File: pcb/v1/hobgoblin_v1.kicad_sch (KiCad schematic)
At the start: 45 parts, among them J1 5V, J2 RC2014EXT1, J3 RC2014EXT2, SW1 RESET, SW2 ROMBNK, U1 74LS32, U2 Z80CPU, U3 74LS14, U4 74LS138, U5 628128, U6 74LS32, U7 74HCT00, U8 SST39SF010, U9 MC68B50, X1 10MHz, X2 7.3728MHz

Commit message: Rename CF Card connector footprint to match the actual part
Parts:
- CF1: footprint hobgoblin:CF-Card_3M_N7E50-7516PK-20-WF -> hobgoblin:CF-Card_3M_N7E507516PK20
- U1: footprint (none) -> Package_DIP:DIP-14_W7.62mm_LongPads
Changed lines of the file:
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@@
     (property "Reference" "CF1" (id 0) (at 222.25 18.669 0))
     (property "Value" "CF_Socket" (id 1) (at 222.25 20.9804 0))
-    (property "Footprint" "hobgoblin:CF-Card_3M_N7E50-7516PK-20-WF" (id 2) (at 222.25 57.15 0)
+    (property "Footprint" "hobgoblin:CF-Card_3M_N7E507516PK20" (id 2) (at 222.25 57.15 0)
       (effects (font (size 1.27 1.27)) hide)
     )
@@
     (property "Reference" "U1" (id 0) (at 27.94 125.73 0))
     (property "Value" "74LS32" (id 1) (at 33.02 121.92 0))
-    (property "Footprint" "" (id 2) (at 27.94 125.73 0)
+    (property "Footprint" "Package_DIP:DIP-14_W7.62mm_LongPads" (id 2) (at 27.94 125.73 0)
       (effects (font (size 1.27 1.27)) hide)
     )
@@
     )
     (path "/00000000-0000-0000-0000-00005fec22e8"
-      (reference "CF1") (unit 1) (value "CF_Socket") (footprint "hobgoblin:CF-Card_3M_N7E50-7516PK-20-WF")
+      (reference "CF1") (unit 1) (value "CF_Socket") (footprint "hobgoblin:CF-Card_3M_N7E507516PK20")
     )
     (path "/00000000-0000-0000-0000-00005f8c4542"
@@
     )
     (path "/00000000-0000-0000-0000-0000600d80cc"
-      (reference "U1") (unit 2) (value "74LS32") (footprint "")
+      (reference "U1") (unit 2) (value "74LS32") (footprint "Package_DIP:DIP-14_W7.62mm_LongPads")
     )
     (path "/00000000-0000-0000-0000-00005fb5d442"

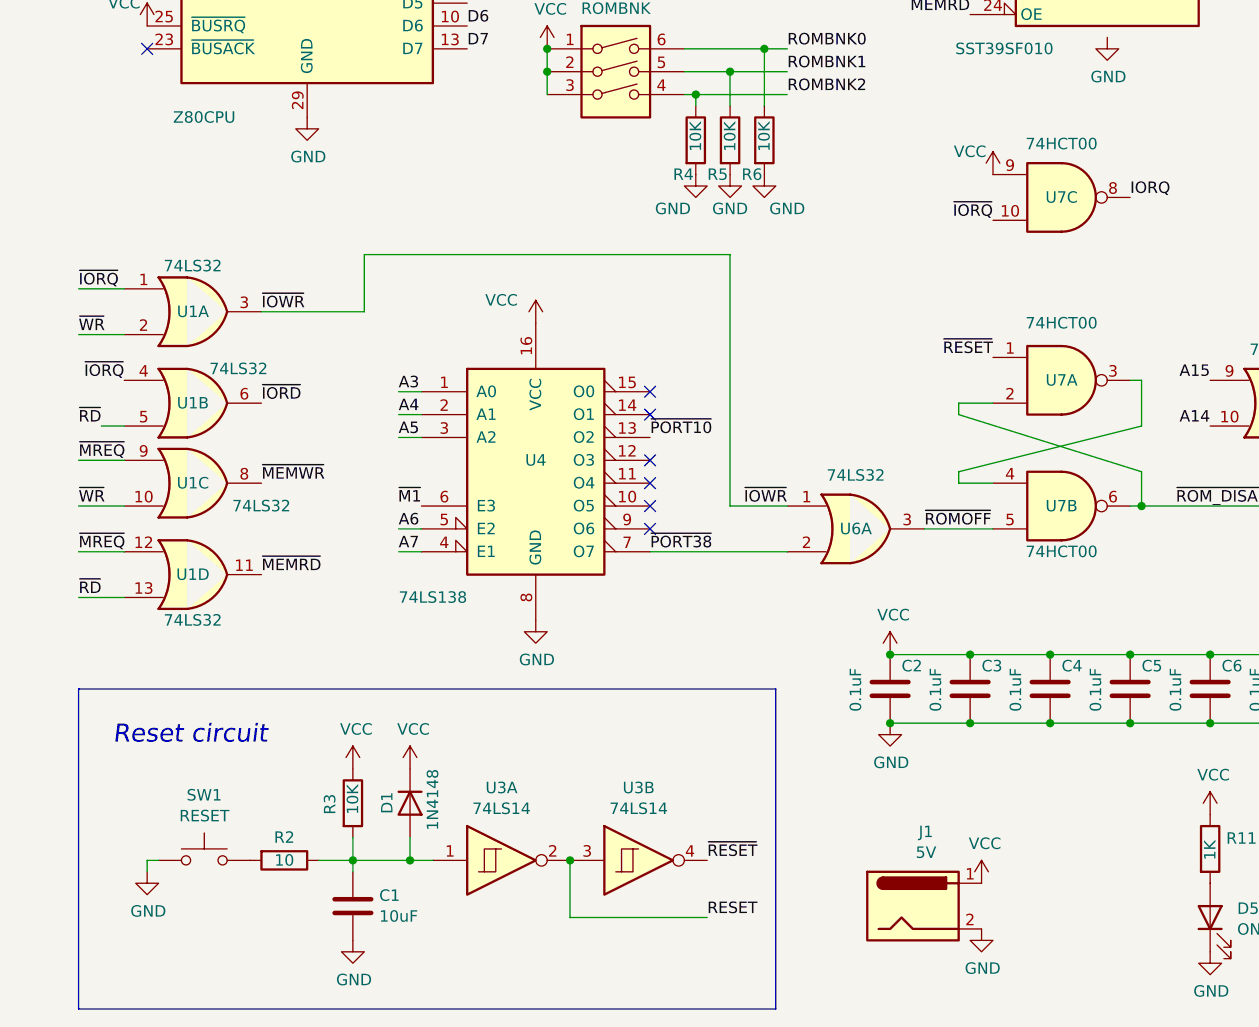
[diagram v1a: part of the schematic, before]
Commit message: Update to latest KiCAD version
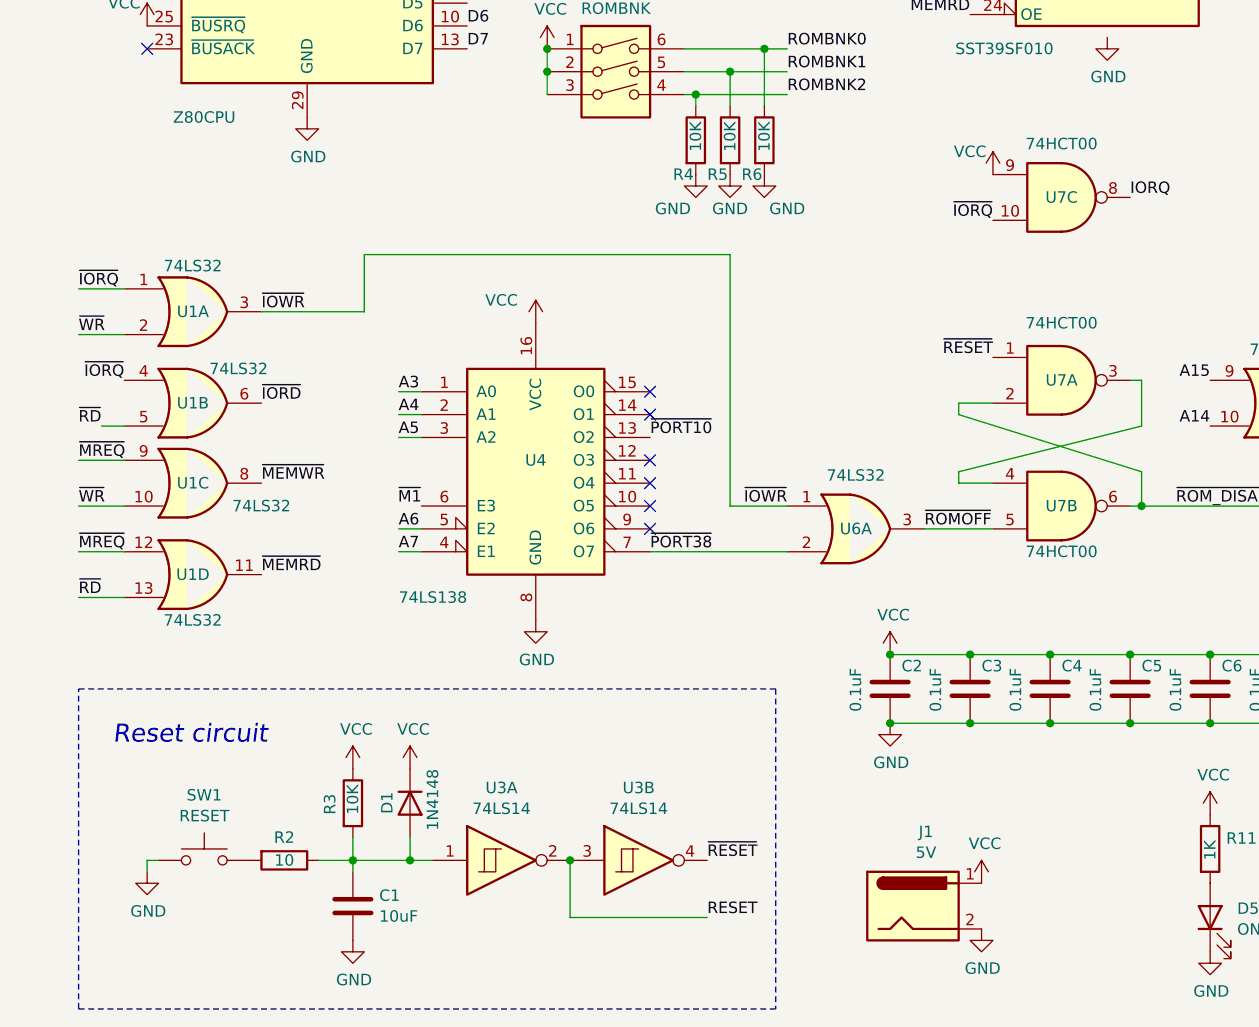
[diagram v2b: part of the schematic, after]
